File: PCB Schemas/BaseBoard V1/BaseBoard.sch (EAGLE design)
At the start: 31 parts, among them IC1 ATMEGA2560AU, J1 PROGRAM, J2 CON06X2-2MM, U1 74HC595D, U2 74HC595D, U3 74HC595D, X1 16MHz

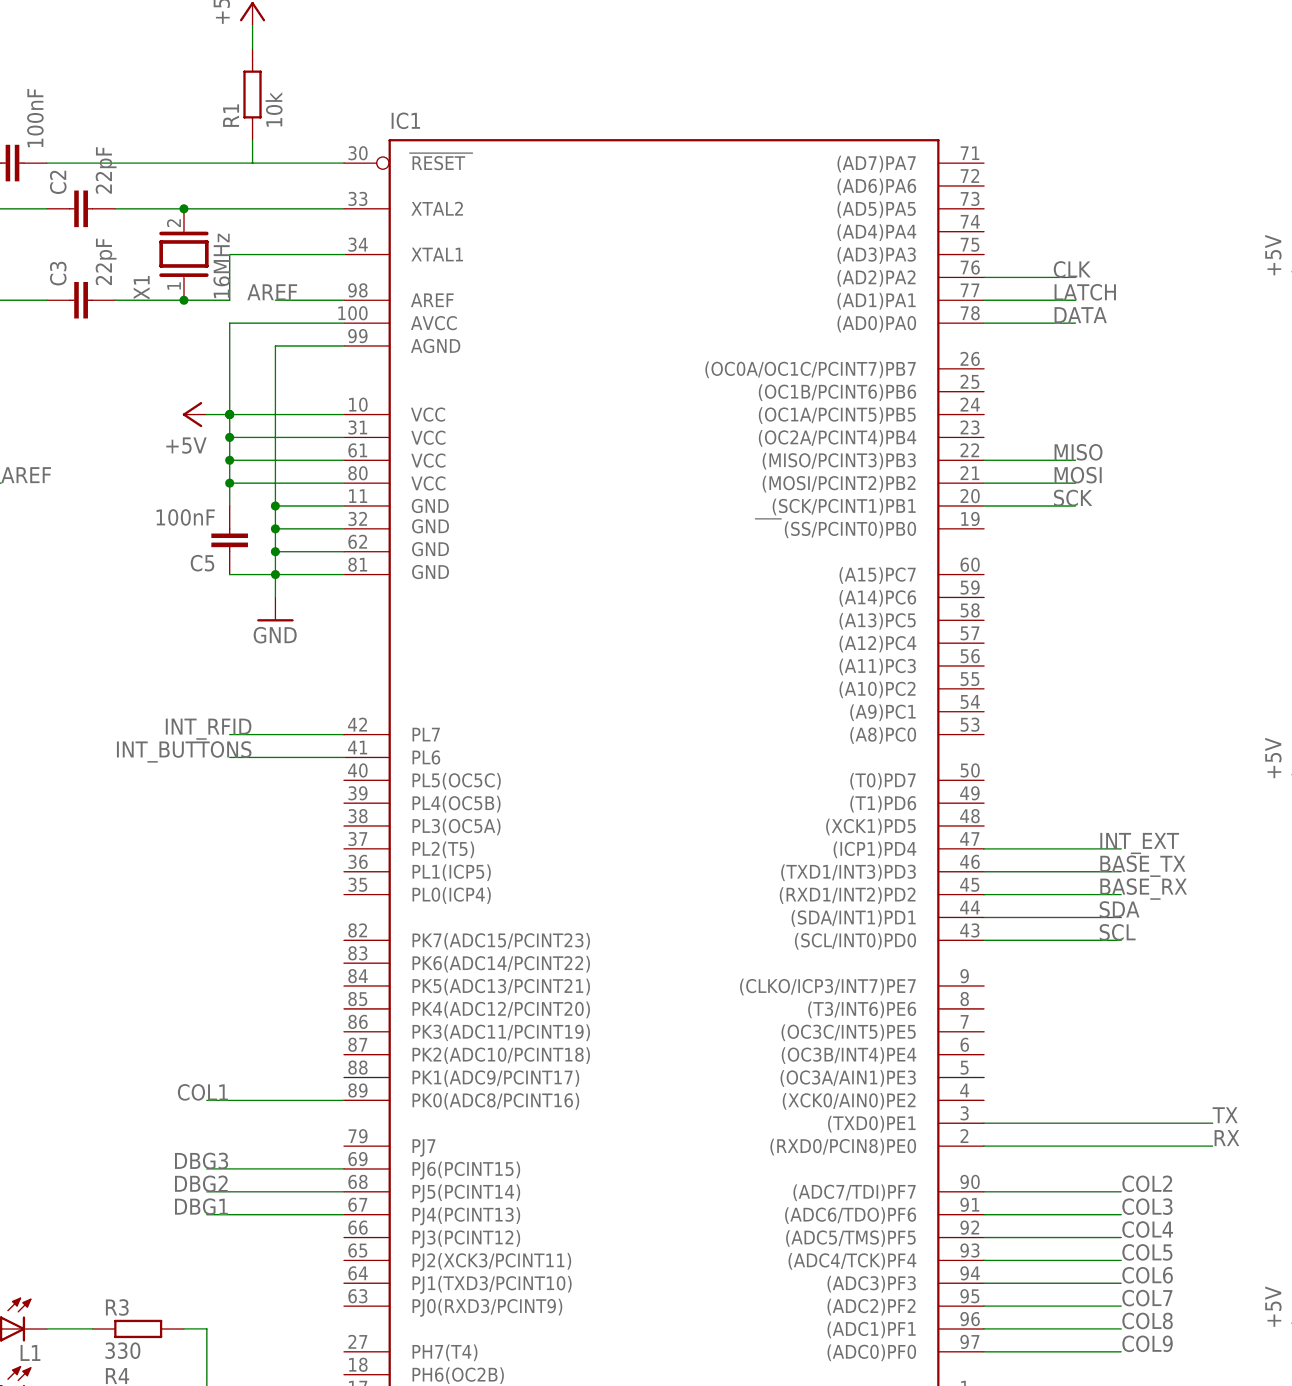
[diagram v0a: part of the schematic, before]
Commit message: Changed debug pins
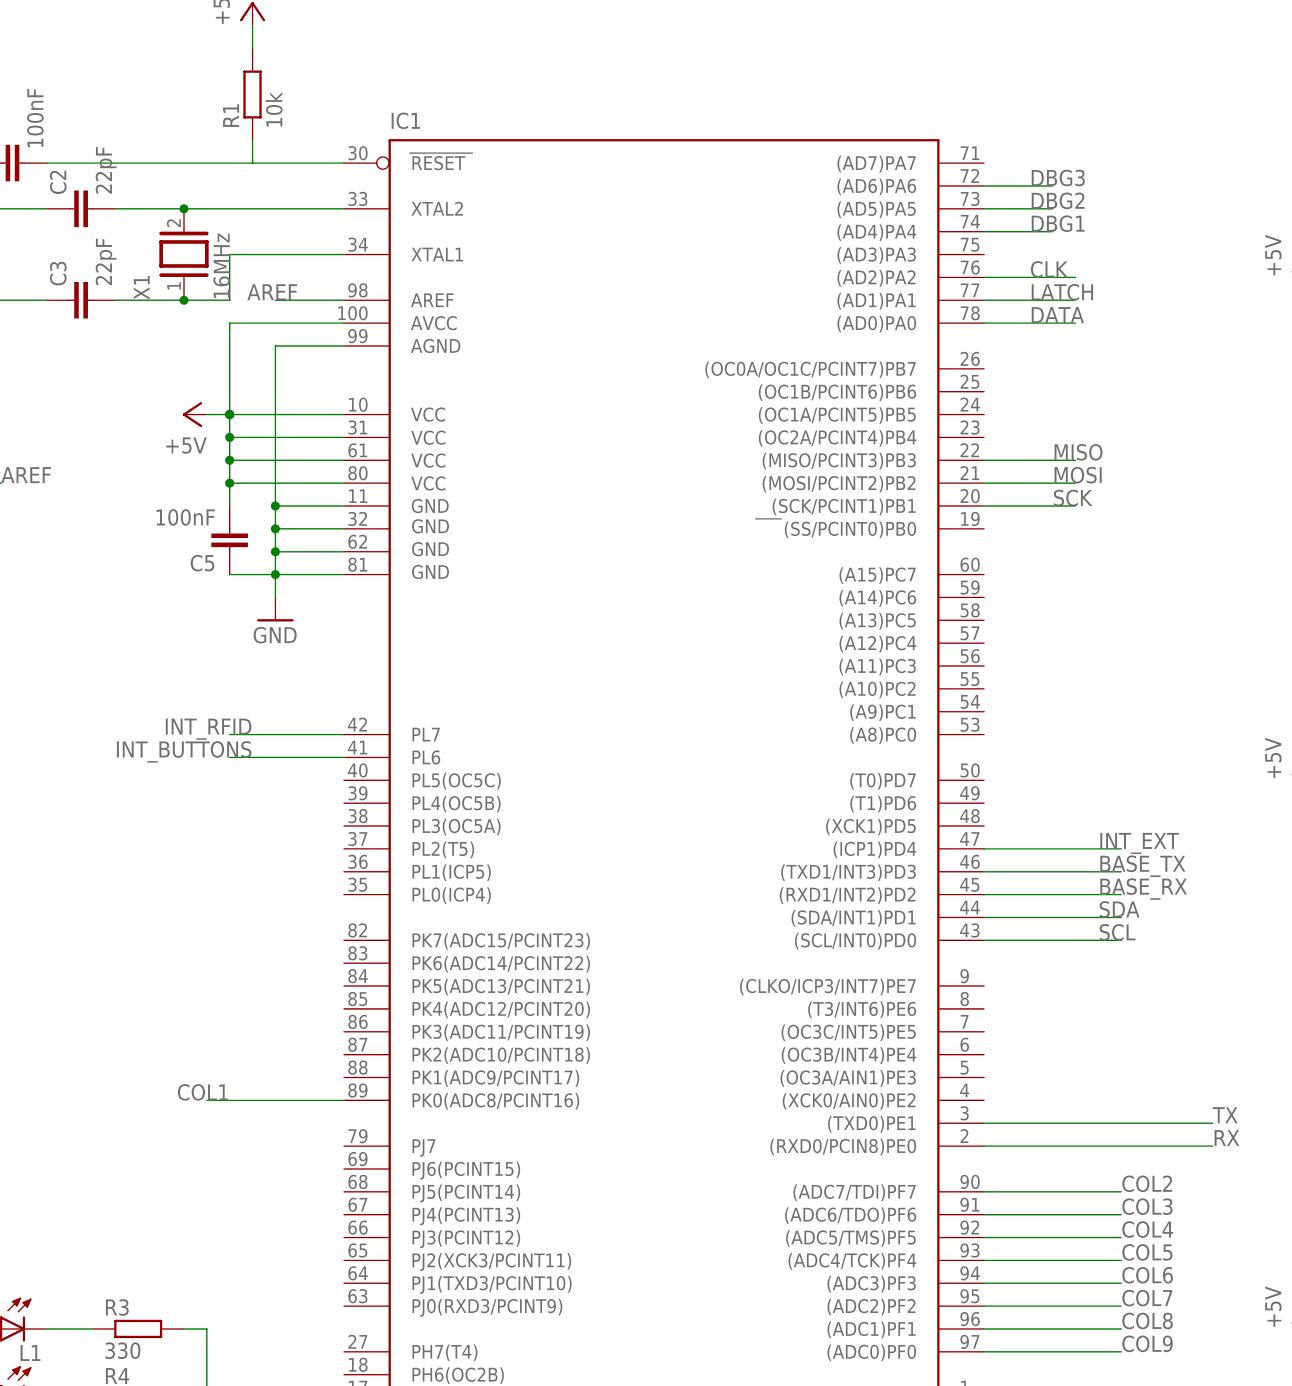
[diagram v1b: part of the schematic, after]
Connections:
- net DBG1: now also IC1.(AD4)PA4; no longer IC1.PJ4(PCINT13)
- net DBG2: now also IC1.(AD5)PA5; no longer IC1.PJ5(PCINT14)
- net DBG3: now also IC1.(AD6)PA6; no longer IC1.PJ6(PCINT15)
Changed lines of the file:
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@@
 <pinref part="IC1" gate="1" pin="(AD0)PA0"/>
 <wire x1="106.68" y1="88.9" x2="116.84" y2="88.9" width="0.1524" layer="91"/>
-<label x="114.3" y="88.9" size="1.778" layer="95"/>
+<label x="111.76" y="88.9" size="1.778" layer="95"/>
 </segment>
 </net>
@@
 <pinref part="IC1" gate="1" pin="(AD2)PA2"/>
 <wire x1="106.68" y1="93.98" x2="116.84" y2="93.98" width="0.1524" layer="91"/>
-<label x="114.3" y="93.98" size="1.778" layer="95"/>
+<label x="111.76" y="93.98" size="1.778" layer="95"/>
 </segment>
 </net>
@@
 <pinref part="IC1" gate="1" pin="(AD1)PA1"/>
 <wire x1="106.68" y1="91.44" x2="116.84" y2="91.44" width="0.1524" layer="91"/>
-<label x="114.3" y="91.44" size="1.778" layer="95"/>
+<label x="111.76" y="91.44" size="1.778" layer="95"/>
 </segment>
 </net>
@@
 </segment>
 <segment>
-<pinref part="IC1" gate="1" pin="PJ5(PCINT14)"/>
-<wire x1="35.56" y1="-7.62" x2="20.32" y2="-7.62" width="0.1524" layer="91"/>
-<label x="22.86" y="-7.62" size="1.778" layer="95" rot="MR0"/>
+<pinref part="IC1" gate="1" pin="(AD5)PA5"/>
+<wire x1="106.68" y1="101.6" x2="114.3" y2="101.6" width="0.1524" layer="91"/>
+<label x="111.76" y="101.6" size="1.778" layer="95"/>
 </segment>
 </net>
@@
 </segment>
 <segment>
-<pinref part="IC1" gate="1" pin="PJ6(PCINT15)"/>
-<wire x1="35.56" y1="-5.08" x2="20.32" y2="-5.08" width="0.1524" layer="91"/>
-<label x="22.86" y="-5.08" size="1.778" layer="95" rot="MR0"/>
+<pinref part="IC1" gate="1" pin="(AD6)PA6"/>
+<wire x1="106.68" y1="104.14" x2="114.3" y2="104.14" width="0.1524" layer="91"/>
+<label x="111.76" y="104.14" size="1.778" layer="95"/>
 </segment>
 </net>
@@
 </segment>
 <segment>
-<pinref part="IC1" gate="1" pin="PJ4(PCINT13)"/>
-<wire x1="35.56" y1="-10.16" x2="20.32" y2="-10.16" width="0.1524" layer="91"/>
-<label x="22.86" y="-10.16" size="1.778" layer="95" rot="MR0"/>
-</segment>
-</net>
+<pinref part="IC1" gate="1" pin="(AD4)PA4"/>
+<wire x1="106.68" y1="99.06" x2="114.3" y2="99.06" width="0.1524" layer="91"/>
+<label x="111.76" y="99.06" size="1.778" layer="95"/>
+</segment>
+</net>

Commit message: Revert "Changed debug pins"
This reverts commit 73787cc4df0c0002b7e389e6993c433356a097db.
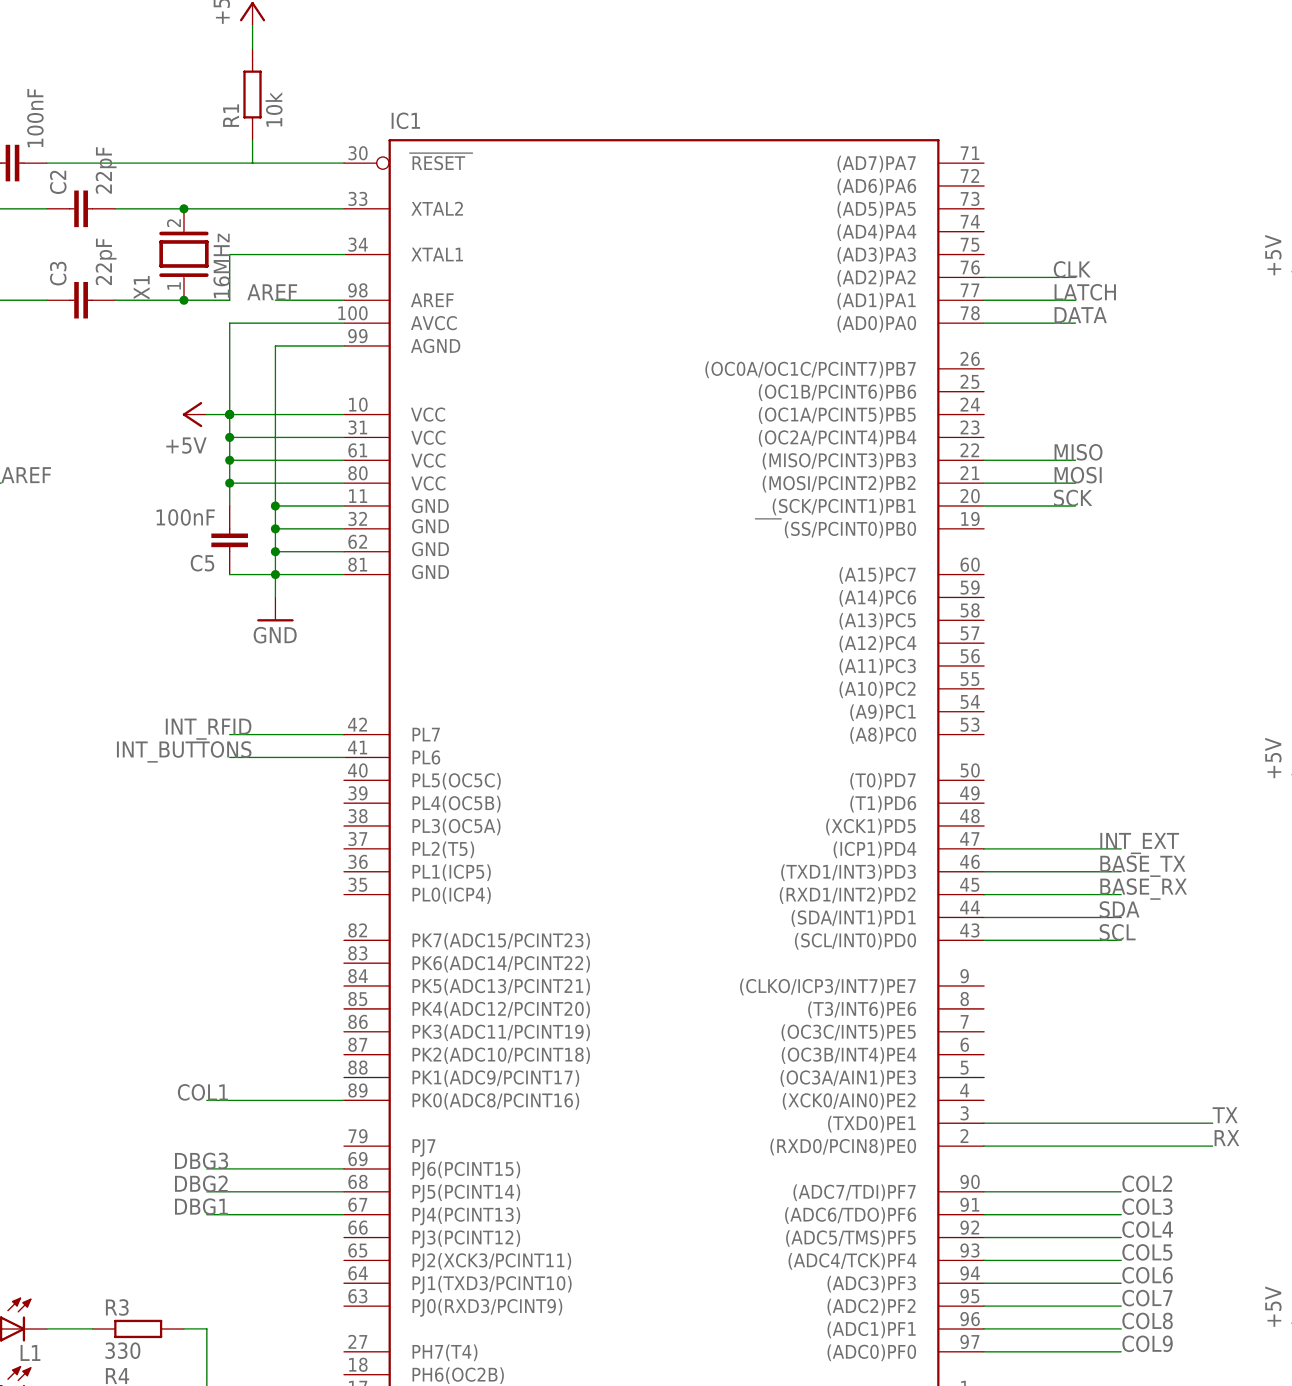
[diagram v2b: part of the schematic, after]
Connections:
- net DBG1: now also IC1.PJ4(PCINT13); no longer IC1.(AD4)PA4
- net DBG2: now also IC1.PJ5(PCINT14); no longer IC1.(AD5)PA5
- net DBG3: now also IC1.PJ6(PCINT15); no longer IC1.(AD6)PA6
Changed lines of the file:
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@@
 <pinref part="IC1" gate="1" pin="(AD0)PA0"/>
 <wire x1="106.68" y1="88.9" x2="116.84" y2="88.9" width="0.1524" layer="91"/>
-<label x="111.76" y="88.9" size="1.778" layer="95"/>
+<label x="114.3" y="88.9" size="1.778" layer="95"/>
 </segment>
 </net>
@@
 <pinref part="IC1" gate="1" pin="(AD2)PA2"/>
 <wire x1="106.68" y1="93.98" x2="116.84" y2="93.98" width="0.1524" layer="91"/>
-<label x="111.76" y="93.98" size="1.778" layer="95"/>
+<label x="114.3" y="93.98" size="1.778" layer="95"/>
 </segment>
 </net>
@@
 <pinref part="IC1" gate="1" pin="(AD1)PA1"/>
 <wire x1="106.68" y1="91.44" x2="116.84" y2="91.44" width="0.1524" layer="91"/>
-<label x="111.76" y="91.44" size="1.778" layer="95"/>
+<label x="114.3" y="91.44" size="1.778" layer="95"/>
 </segment>
 </net>
@@
 </segment>
 <segment>
-<pinref part="IC1" gate="1" pin="(AD5)PA5"/>
-<wire x1="106.68" y1="101.6" x2="114.3" y2="101.6" width="0.1524" layer="91"/>
-<label x="111.76" y="101.6" size="1.778" layer="95"/>
+<pinref part="IC1" gate="1" pin="PJ5(PCINT14)"/>
+<wire x1="35.56" y1="-7.62" x2="20.32" y2="-7.62" width="0.1524" layer="91"/>
+<label x="22.86" y="-7.62" size="1.778" layer="95" rot="MR0"/>
 </segment>
 </net>
@@
 </segment>
 <segment>
-<pinref part="IC1" gate="1" pin="(AD6)PA6"/>
-<wire x1="106.68" y1="104.14" x2="114.3" y2="104.14" width="0.1524" layer="91"/>
-<label x="111.76" y="104.14" size="1.778" layer="95"/>
+<pinref part="IC1" gate="1" pin="PJ6(PCINT15)"/>
+<wire x1="35.56" y1="-5.08" x2="20.32" y2="-5.08" width="0.1524" layer="91"/>
+<label x="22.86" y="-5.08" size="1.778" layer="95" rot="MR0"/>
 </segment>
 </net>
@@
 </segment>
 <segment>
-<pinref part="IC1" gate="1" pin="(AD4)PA4"/>
-<wire x1="106.68" y1="99.06" x2="114.3" y2="99.06" width="0.1524" layer="91"/>
-<label x="111.76" y="99.06" size="1.778" layer="95"/>
-</segment>
-</net>
+<pinref part="IC1" gate="1" pin="PJ4(PCINT13)"/>
+<wire x1="35.56" y1="-10.16" x2="20.32" y2="-10.16" width="0.1524" layer="91"/>
+<label x="22.86" y="-10.16" size="1.778" layer="95" rot="MR0"/>
+</segment>
+</net>
